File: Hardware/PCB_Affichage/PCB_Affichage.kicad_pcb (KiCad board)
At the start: 2 copper layers, 34 x 27 mm, 1 part

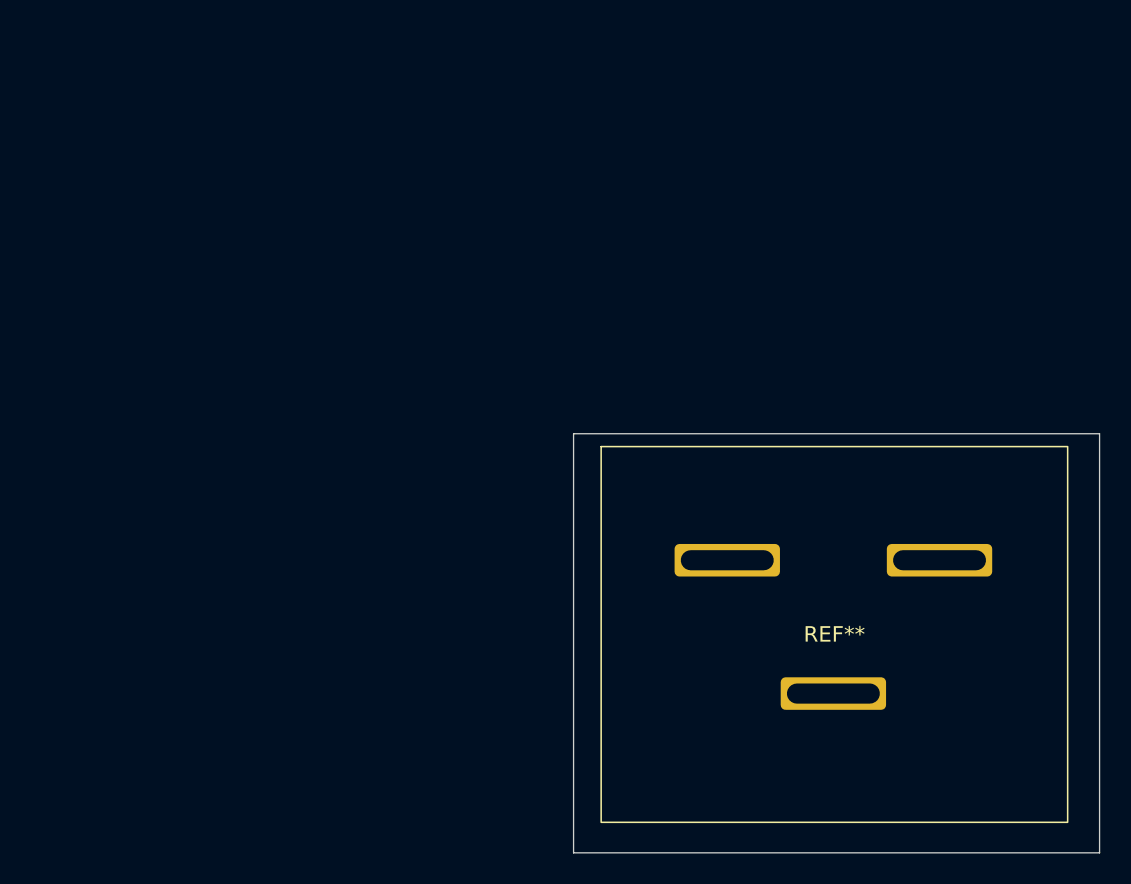
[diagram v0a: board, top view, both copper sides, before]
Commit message: finalisation PCB affichage
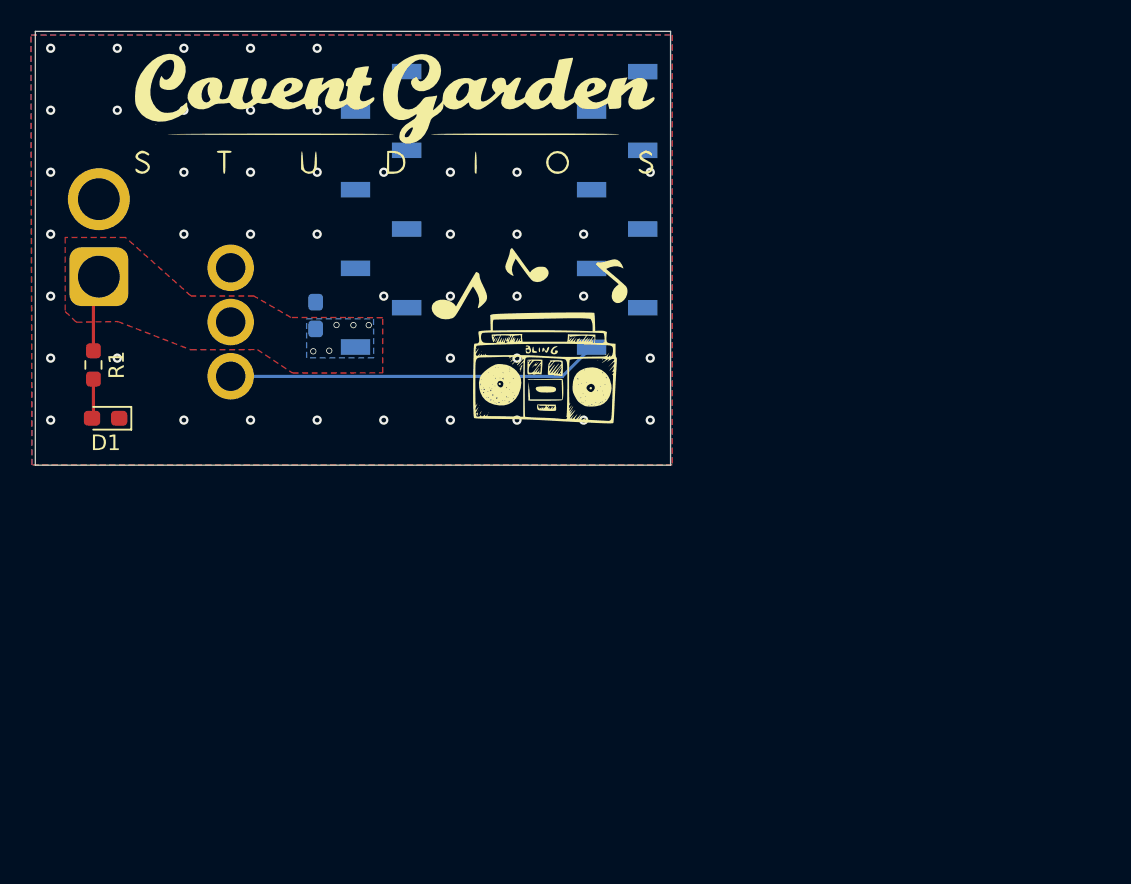
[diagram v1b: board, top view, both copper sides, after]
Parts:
- removed REF**: Conn_Secteur_femelle, Conn_secteur:Conn_Secteur_femelle
- added C1: 100n, Capacitor_SMD:C_0603_1608Metric_Pad1.08x0.95mm_HandSolder, B.Cu at (105.1, 64.3)
- added D1: LED, LED_SMD:LED_0603_1608Metric_Pad1.05x0.95mm_HandSolder, F.Cu at (91.5, 71.0)
- added G***: LOGO, img:Logo_Covent, F.Cu at (110.3, 51.7)
- added G***: LOGO, img:Dessin_CoventGarden, F.Cu at (119.4, 66.0)
- added J1: Conn_01x02, Connector_AMASS:AMASS_XT30U-F_1x02_P5.0mm_Vertical, B.Cu at (91.1, 61.8)
- added J2: Conn_01x03, Conn:MR30_F, B.Cu at (99.6, 64.8)
- added R1: 2k5, Resistor_SMD:R_0603_1608Metric_Pad0.98x0.95mm_HandSolder, F.Cu at (90.8, 67.5)
- added U2: ~, ESP32_SuperMini:SuperMini SMT, B.Cu at (116.9, 57.5)
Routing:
- net /Px: track 0.00 -> 24.1 mm
- net +5V: track 0.00 -> 4.93 mm, vias 0 -> 5
- net Net-(D1-A): track 0.00 -> 2.57 mm
- net GND: vias 0 -> 44
- added copper zone on B.Cu, net +5V
- added copper zone on F.Cu, net +5V
- added copper zone on B.Cu, net GND
- added copper zone on F.Cu, net GND
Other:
- board size 34 x 27 mm -> 41 x 28 mm
- board text added: "By Capodagli Janus"
